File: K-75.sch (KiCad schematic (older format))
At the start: 193 parts, among them J1 Conn_01x04, SW1 SW_Push, U1 ATmega32U4-AU, Y1 Crystal_GND24_Small

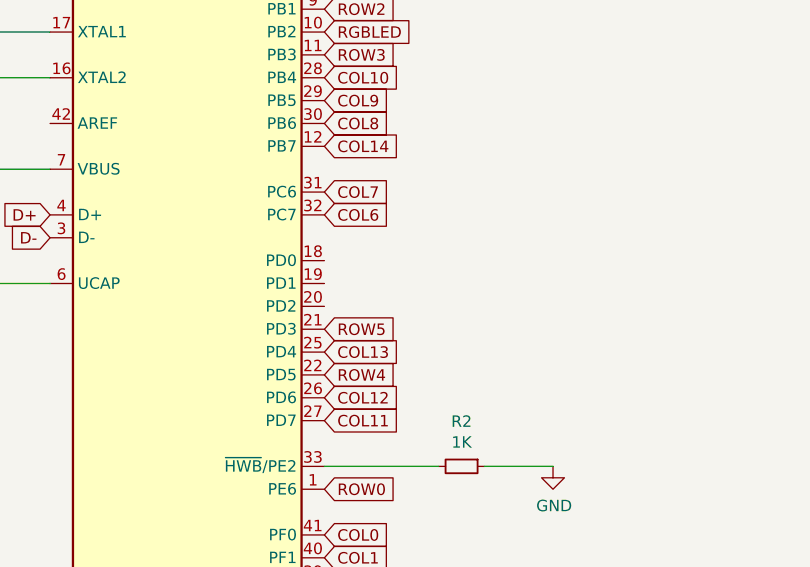
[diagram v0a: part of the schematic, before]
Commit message: Finished traces
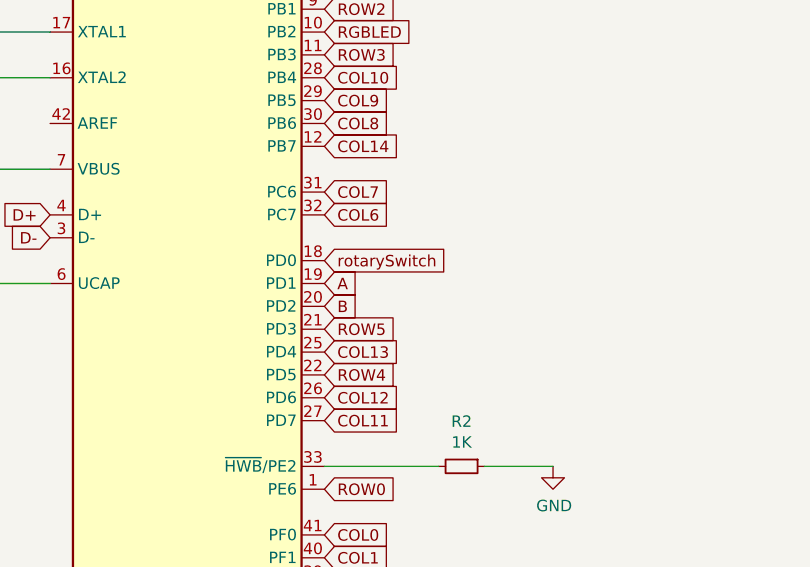
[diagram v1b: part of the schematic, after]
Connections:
- net rotarySwitch: now reaches U1.18 (PD0)
- net A: now reaches U1.19 (PD1)
- net B: now reaches U1.20 (PD2)
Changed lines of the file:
@@
 COL14
 $Comp
-L power:+5V #PWR?
+L power:+5V #PWR0112
 U 1 1 62738D63
 P 5900 10800
-F 0 "#PWR?" H 5900 10650 50  0001 C CNN
+F 0 "#PWR0112" H 5900 10650 50  0001 C CNN
 F 1 "+5V" H 5915 10973 50  0000 C CNN
 F 2 "" H 5900 10800 50  0001 C CNN
@@
 	1    0    0    -1
 $EndComp
+Text GLabel 4750 8450 2    50   Input ~ 0
+rotarySwitch
+Text GLabel 4750 8550 2    50   Input ~ 0
+A
+Text GLabel 4750 8650 2    50   Input ~ 0
+B
 $EndSCHEMATC
